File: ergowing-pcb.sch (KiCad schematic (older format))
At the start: 16 parts, among them J1 USB_mini_micro_B, SW1 SW_PUSH, U1 ATMEGA32U4, X1 XTAL_GND

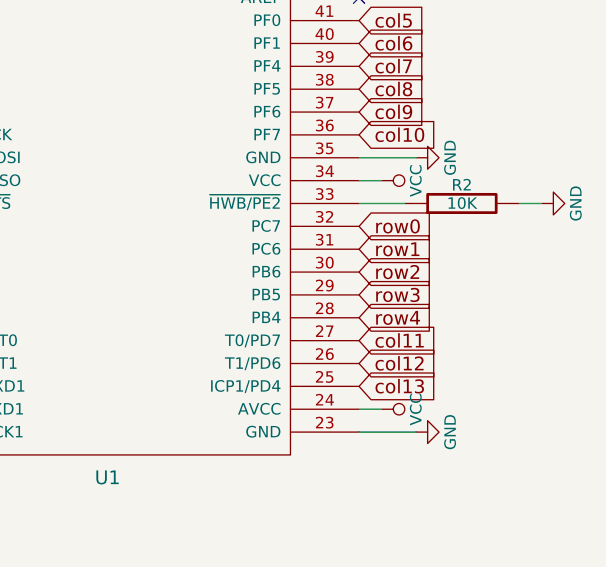
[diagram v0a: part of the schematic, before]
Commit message: Pre-messing around #1
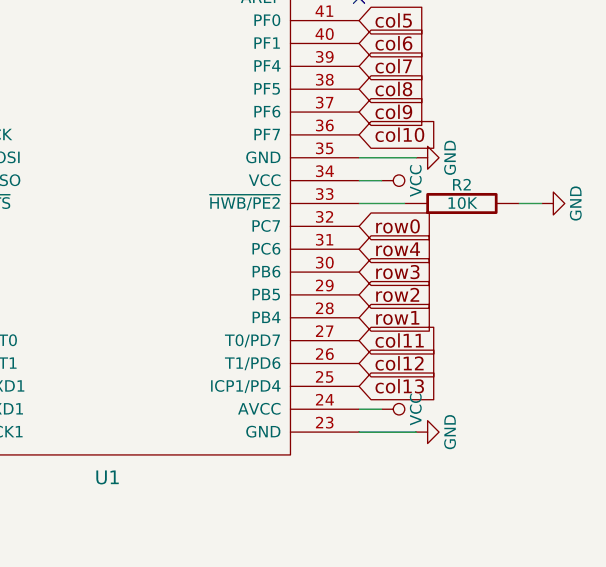
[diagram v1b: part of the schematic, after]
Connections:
- net row1: now also U1.28 (PB4); no longer U1.31 (PC6)
- net row2: now also U1.29 (PB5); no longer U1.30 (PB6)
- net row3: now also U1.30 (PB6); no longer U1.29 (PB5)
- net row4: now also U1.31 (PC6); no longer U1.28 (PB4)
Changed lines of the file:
@@
 row0
 Text GLabel 4600 3950 2    60   Input ~ 0
+row4
+Text GLabel 4600 4050 2    60   Input ~ 0
+row3
+Text GLabel 4600 4150 2    60   Input ~ 0
+row2
+Text GLabel 4600 4250 2    60   Input ~ 0
 row1
-Text GLabel 4600 4050 2    60   Input ~ 0
-row2
-Text GLabel 4600 4150 2    60   Input ~ 0
-row3
-Text GLabel 4600 4250 2    60   Input ~ 0
-row4
 Text GLabel 2450 3650 0    60   Input ~ 0
 col0
